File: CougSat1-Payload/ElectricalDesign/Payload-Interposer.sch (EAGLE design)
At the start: 62 parts, among them J1 CougSat Card, J3 Interposer, J5 Germination Chamber, Q1 CSD25402Q3A, Q2 CSD25402Q3A, U1 TXS0102DQM, U14 TPS61220, U15 TPS73250, U2 TXS0102DQM, U3 TXS0102DQM, U4 BME280, U5 TLC59116F, U6 TXS0102DQM

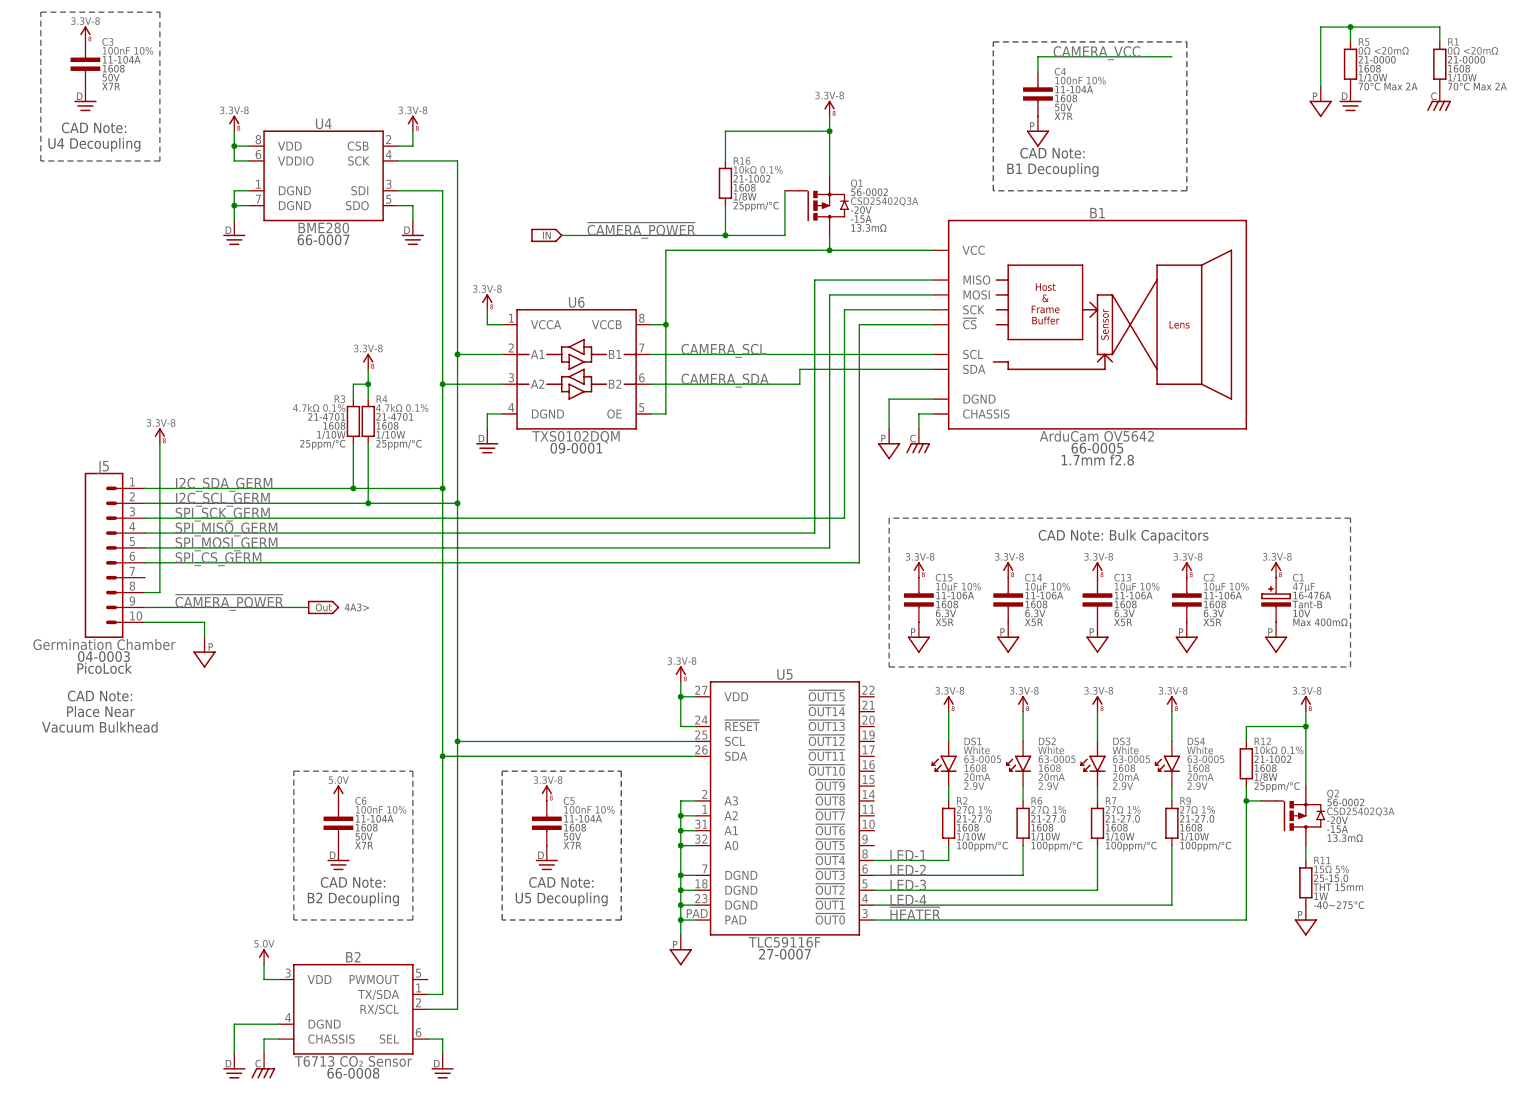
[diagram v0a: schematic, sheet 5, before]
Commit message: Worked on layout
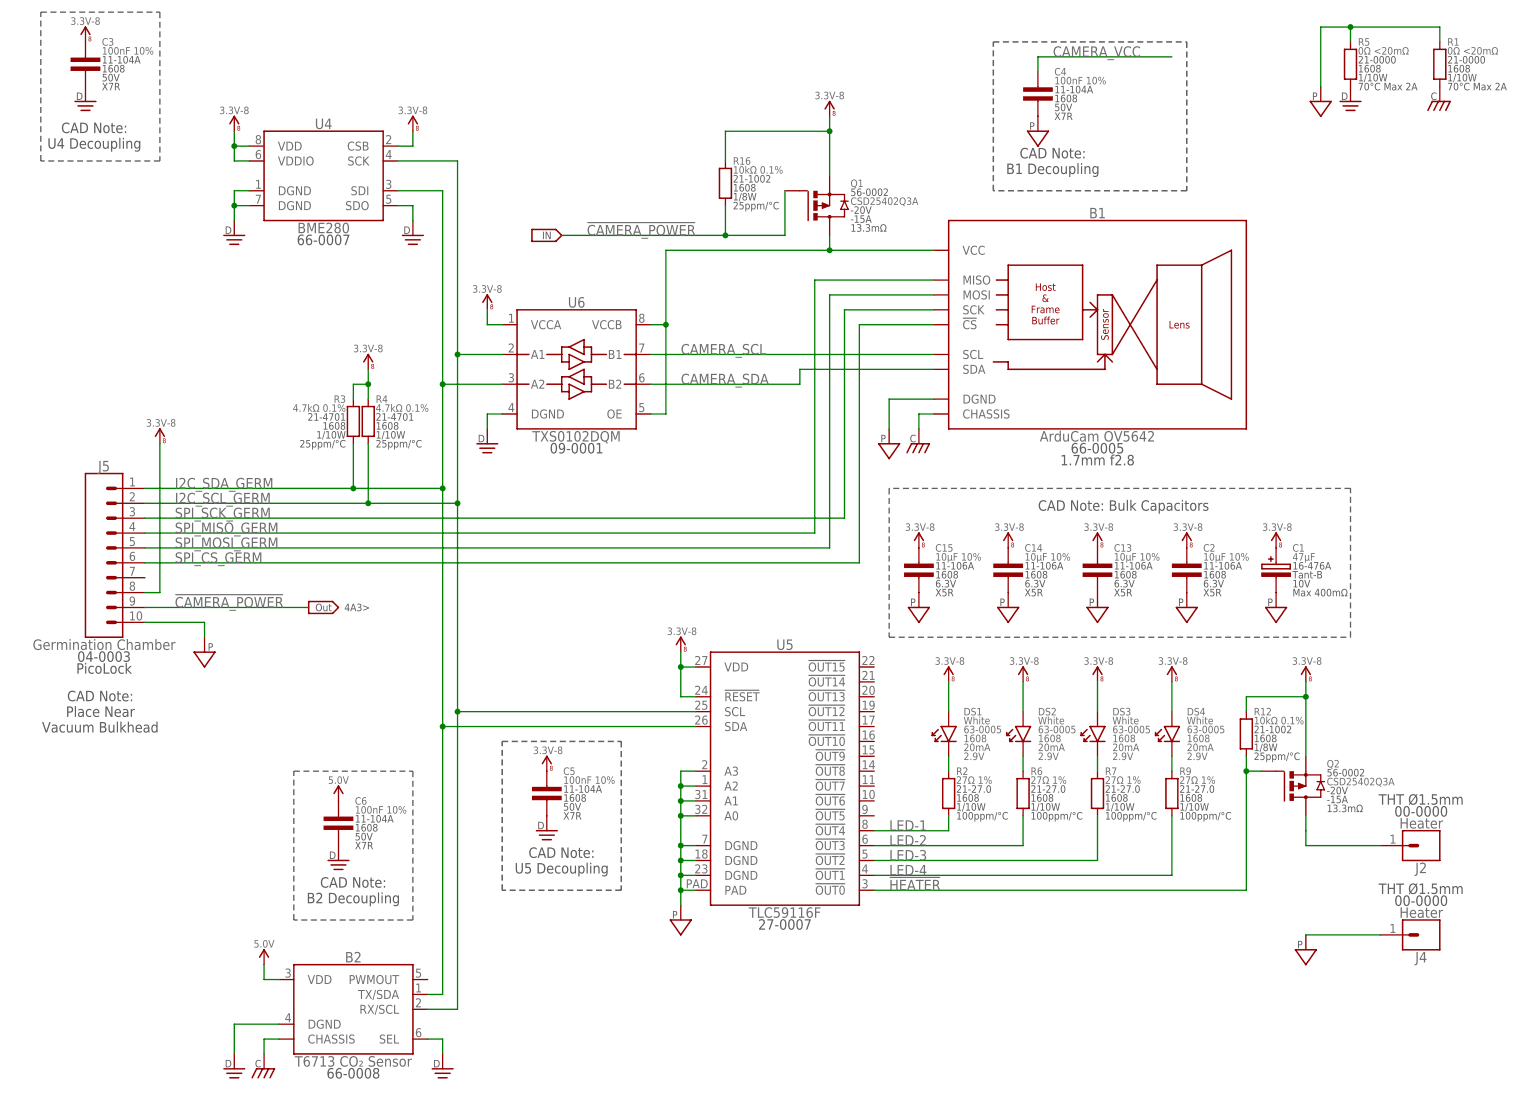
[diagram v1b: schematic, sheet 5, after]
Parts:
- removed R11: 15Ω 5%, CougsInSpace-Resistors:RES-V-15R-THT-15MM
- added J2, J4: Heater, CougsInSpace-Connectors:1X01-THT-1.5
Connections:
- net HEATER_SOURCE: now also J2.1; no longer R11.2
- net PGND: now also J4.1; no longer R11.1
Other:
- moved on the sheet: C1, C13, C14, C15, C2, C5, DS1, DS2, DS3, DS4, Q2, R12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
